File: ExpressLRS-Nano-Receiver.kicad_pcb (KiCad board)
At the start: 4 copper layers, 17 x 12 mm, 38 parts, among them J1 CONN, U1 TPS73533DRVR, U2 ESP8285, U3 SX1280IMLTRT, Y1 26MHz, Y2 52MHz

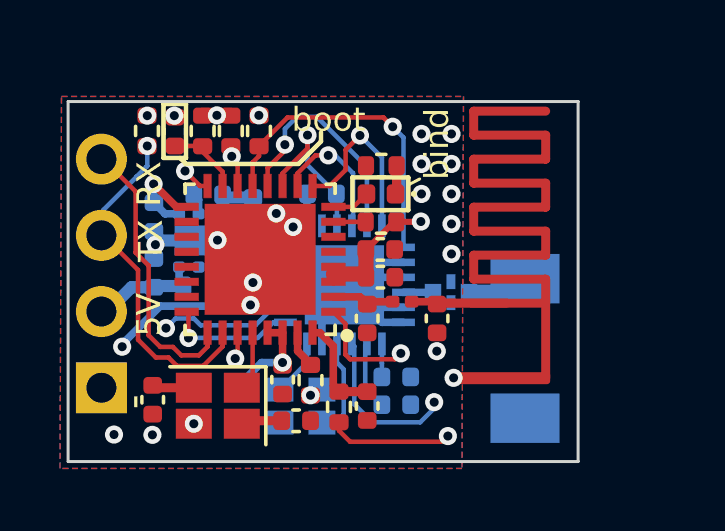
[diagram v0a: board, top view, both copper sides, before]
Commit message: update
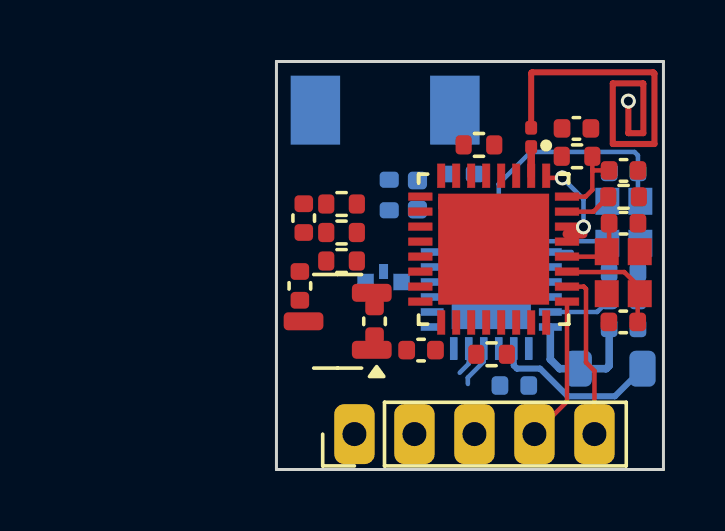
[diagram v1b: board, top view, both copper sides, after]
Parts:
- removed AE1: Antenna_Dipole, Library:esp-antenna
- removed C12, C19, C9: ~, Capacitor_SMD:C_0402_1005Metric
- removed C16: 470nF, Capacitor_SMD:C_0402_1005Metric
- removed C7: 4.7uF, Capacitor_SMD:C_0402_1005Metric
- removed R7: 100K, Resistor_SMD:R_0402_1005Metric
- removed U1: TPS73533DRVR, Package_SON:WSON-6-1EP_2x2mm_P0.65mm_EP1x1.6mm
- added C20: 2.2uF, Capacitor_SMD:C_0402_1005Metric, F.Cu at (99.9, 63.8)
- added C21: 2.2uF, Capacitor_SMD:C_0402_1005Metric, F.Cu at (102.4, 65.0)
- added L1: 15uH, Inductor_SMD:L_0805_2012Metric, B.Cu at (110.3, 66.6)
- added U4: AP2210N-3.3TRG1, Package_TO_SOT_SMD:SOT-23-3, F.Cu at (101.2, 65.0)
- C1: value 2.2uF -> 470nF
- C17, C8: moved to F.Cu
- C2: value 10nF -> 18pF
- C5: value 0.1uF -> 18pF
- C6, D1, R9: moved to B.Cu
- J1: value CONN -> Conn_01x05_Pin; footprint Connector_PinHeader_2.54mm:PinHeader_1x04_P2.54mm_Vertical -> Connector_PinHeader_2.00mm:PinHeader_1x05_P2.00mm_Vertical
- Y1: footprint Crystal:Crystal_SMD_EuroQuartz_X22-4Pin_2.5x2.0mm -> Crystal:Crystal_SMD_2016-4Pin_2.0x1.6mm
- moved C10 16.8 mm to (110.7, 61.7), turned to 0 degrees
- moved C1 16.1 mm to (110.7, 65.2), turned to 0 degrees
- moved C5 15.7 mm to (110.7, 63.4), turned to 180 degrees
- moved Y1 14.2 mm to (110.7, 63.4), turned to -90 degrees
- moved C2 13.9 mm to (110.7, 60.0)
- moved R8 13.7 mm to (106.3, 66.1), turned to 180 degrees
- moved Y2 12.4 mm to (110.7, 61.7), turned to 90 degrees
- moved R5 12.1 mm to (110.7, 60.8), turned to 0 degrees
- moved C17 11.7 mm to (109.2, 58.6), turned to 0 degrees
- moved C3 11.6 mm to (110.7, 60.0), turned to 180 degrees
- moved R3 11.5 mm to (109.2, 59.5), turned to 180 degrees
- moved C13 11.4 mm to (110.7, 65.0), turned to 180 degrees
- moved C18 10.7 mm to (110.7, 64.3), turned to 0 degrees
- moved E1 9.21 mm to (102.8, 58.0), turned to 0 degrees
- moved J1 8.58 mm to (101.8, 68.8), turned to 90 degrees
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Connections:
- C1 pad 1: GND -> /V_DCC
- C1 pad 2: +3V3 -> GND
- C10 pad 1: Net-(C10-Pad1) -> Net-(U2-XTAL_IN)
- C13 pad 1: Net-(C13-Pad1) -> Net-(U2-XTAL_OUT)
- C15 pad 2: Net-(U3-VDD_INN) -> /V_DCC
- C2 pad 1: Net-(U1-NR/FB) -> GND
- C2 pad 2: GND -> Net-(U3-XTA)
- C5 pad 1: +5V -> GND
- C5 pad 2: GND -> Net-(U3-XTB)
- J1 pad 1: GND -> /BTN
- J1 pad 2: +5V -> GND
- J1 pad 3: /TX -> +5V
- U3 pad 12: Net-(U3-DCC_FB) -> /V_DCC
- U3 pad 14: unconnected-(U3-DCC_SW-Pad14) -> /V_DCC2
- U3 pad 2: Net-(U3-VDD_INN) -> /V_DCC
- Y1 pad 2: Net-(C10-Pad1) -> GND
- Y1 pad 4: Net-(C13-Pad1) -> GND
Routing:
- net +3V3: track 32.9 -> 6.13 mm, vias 9 -> 2
- net /nRST: track 19.3 -> 0.00 mm, vias 2 -> 0
- net GND: track 18.7 -> 0.00 mm, vias 21 -> 0
- net Net-(AE1-Pad1): track 3.21 -> 16.0 mm, vias 0 -> 1
- net /DIO1: track 10.9 -> 0.00 mm, vias 2 -> 0
- net /NSS: track 10.6 -> 0.00 mm, vias 1 -> 0
- net /MOSI: track 7.69 -> 0.93 mm, vias 1 -> 0
- net /SCK: track 5.98 -> 0.00 mm, vias 1 -> 0
- net /TX: track 11.5 -> 5.62 mm, vias 1 -> 0
- net /V_DCC2: track 0.00 -> 5.66 mm
- net Net-(U3-XTA): track 3.28 -> 8.24 mm
- net /V_DCC: track 0.00 -> 4.47 mm
- net /RX: track 9.32 -> 5.53 mm
- net /BUSY: track 4.34 -> 0.71 mm, vias 1 -> 0
- net +5V: track 3.58 -> 0.00 mm
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- removed copper zone on In1.Cu, net +3V3
- removed copper zone on B.Cu, net GND
- removed copper zone on F.Cu, net GND
- removed copper zone on In2.Cu, net GND
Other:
- board size 17 x 12 mm -> 12.9 x 13.6 mm
- board text removed: "-"
- board text removed: "5V"
- board text removed: "ELRS"
- board text removed: "Kolamuc design."
- board text removed: "RX"
- board text removed: "TX"
- board text removed: "V1.0"
- board text removed: "bind"
- board text removed: "boot"
- board text removed: "micro"
